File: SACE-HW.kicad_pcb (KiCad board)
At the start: 2 copper layers, 100 x 100 mm, 188 parts, among them IC1 1769205241, J1 1935161, J10 690-005-299-043, J11 Header_Male_Pin_2.54mm_1X4_,_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, J12 XH-4A connector, J13 XH-4A connector, J14 2350514-8, J15 2350514-8, J16 2350514-8, J17 2350514-8, J18 MEM2075-00-140-01-A, J19 2350514-8, J2 2350514-8, J20 2350514-8, J3 Header_Male_Pin_2.54mm_1X2_,_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, J4 XH-4A connector, J5 Header_Male_Pin_2.54mm_1X6_,_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, J6 691317710003, J7 RF1-01K-D-00-50-BK-HDW, J8 RF1-01K-D-00-50-BK-HDW, J9 1935161, Q1 MCB90N12A-TP, Q2 PMV20XNER, Q3 PMV20XNER, Q4 PMV20XNER, Q5 PMV20XNER, Q6 PMV20XNER, Q7 PMV20XNER, SW1 PTS645SM43SMTR92, SW2 PTS645SM43SMTR92, U1 OKI-78SR-5_1.5-W36H-C, U10 ISO7341CQDWQ1, U11 MCP2221A-I_SL, U12 TLA2528IRTER, U13 TLA2528IRTER, U14 TLV9302IDR, U15 MCP4728T-E_UN, U16 74LVC4245APW_118, U2 AZ1117IH-3.3TRG1, U3 AZ1117IH-3.3TRG1, U4 STM32F446RE, U5 MCP6L04T-E/SL, U6 LTV-816S, U7 LTV-816S, U8 TMCS1101A3UQDT, U9 ADC124S021CIMM

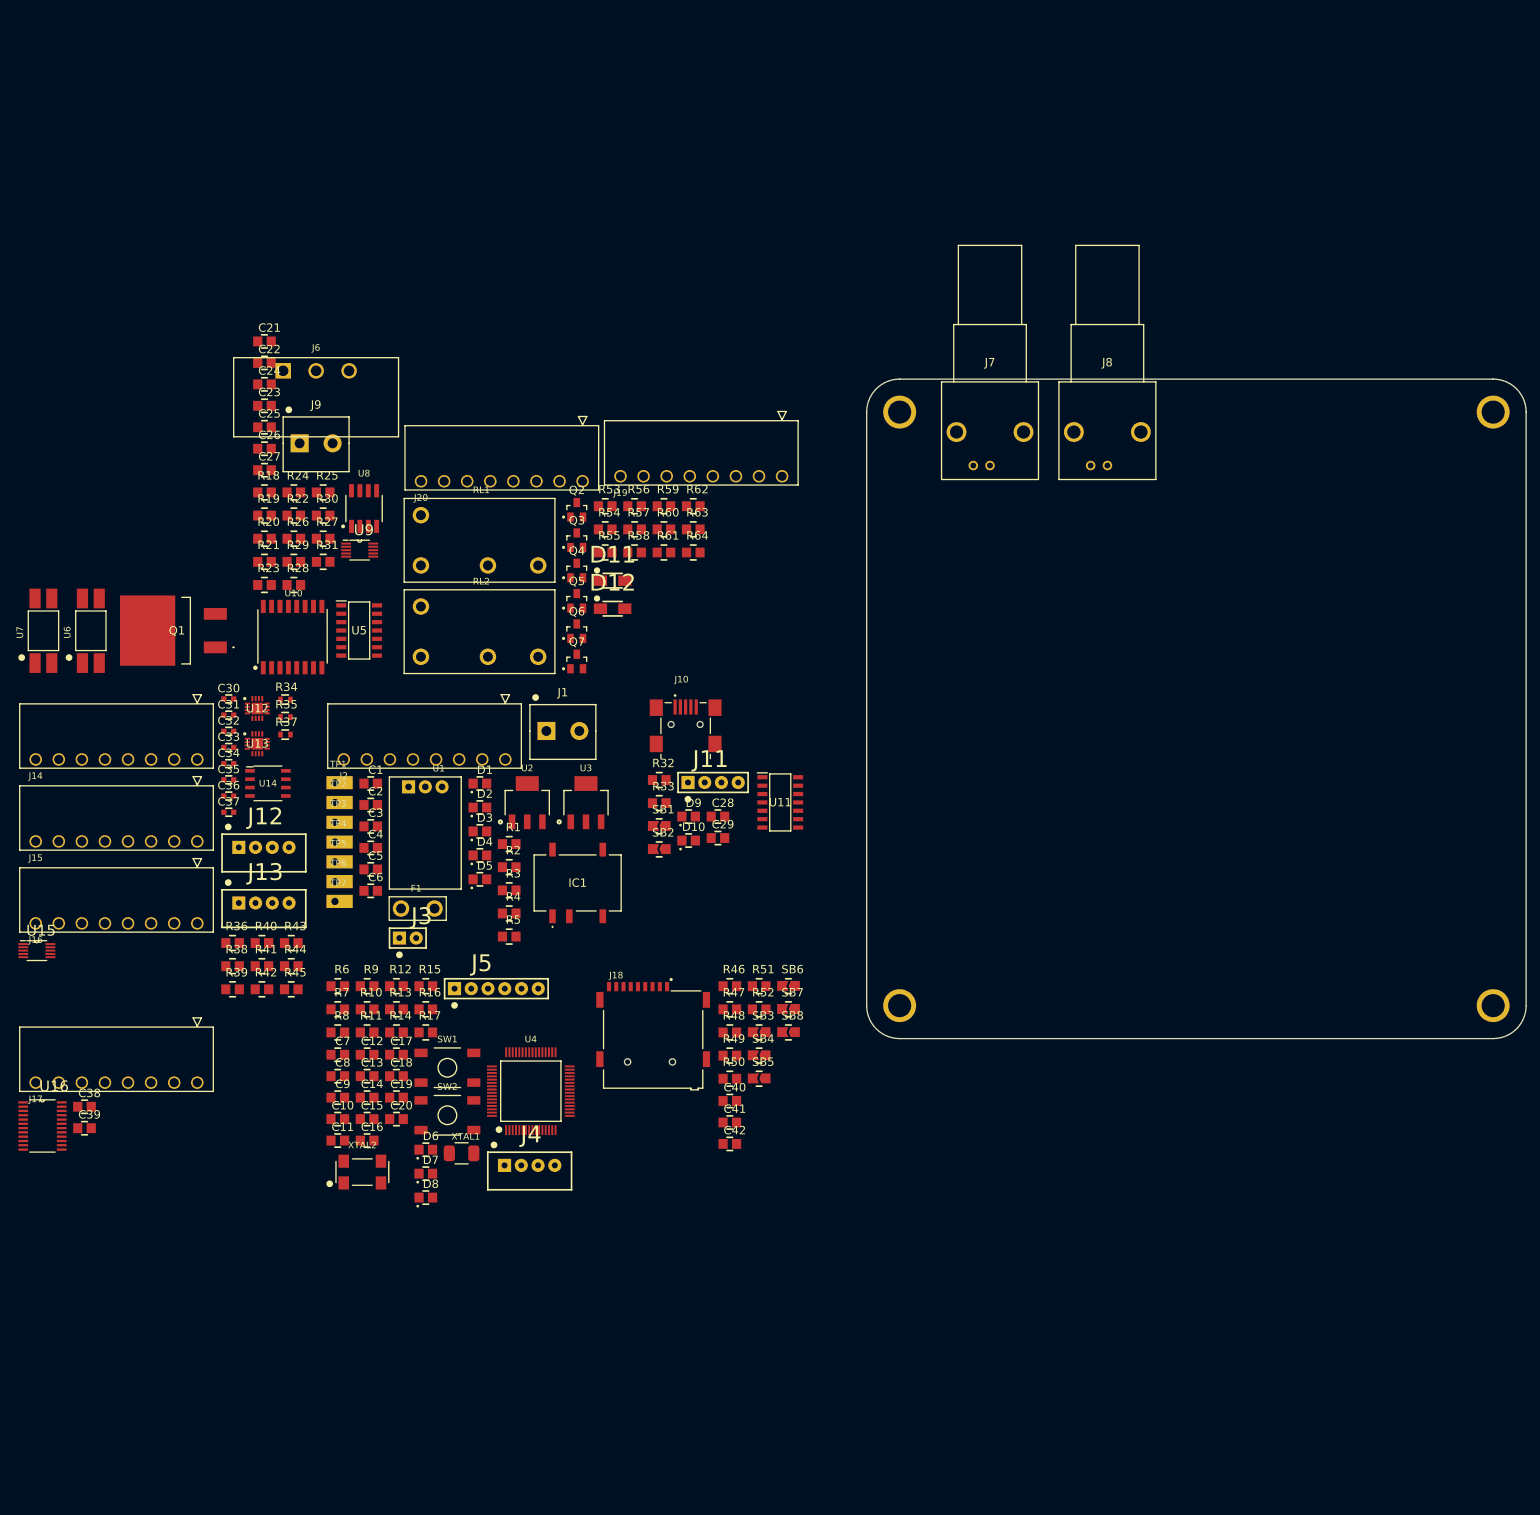
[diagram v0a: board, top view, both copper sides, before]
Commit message: update
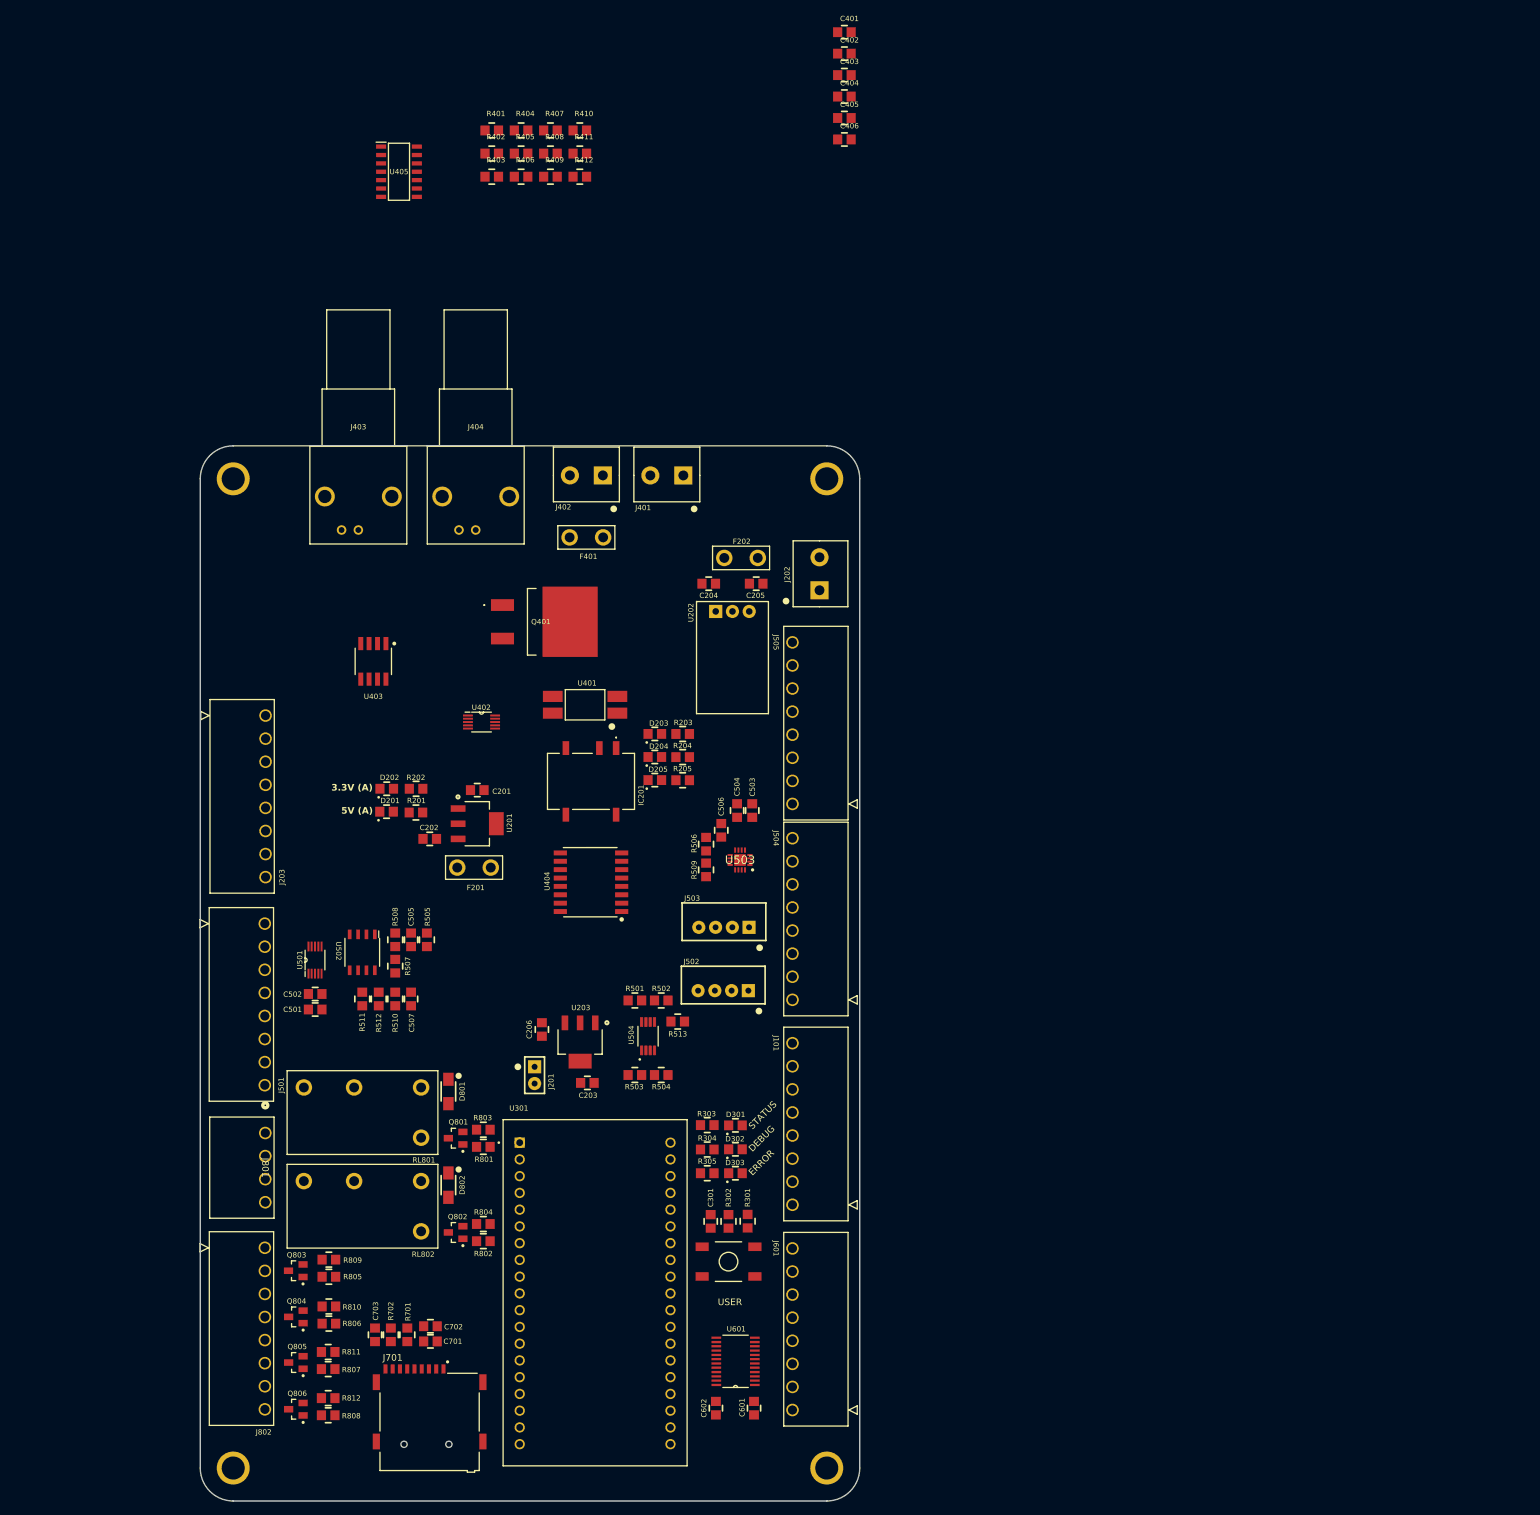
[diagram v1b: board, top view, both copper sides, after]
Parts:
- removed C1, C17, C2: 885012107018, Capacitors:C0805
- removed C10, C13: 885012007027, Capacitors:C0805
- removed C11, C14, C41: 885012107015, Capacitors:C0805
- removed C12: 885012207092, Capacitors:C0805
- removed C15, C16, C18, C19, C20, C22, C23, C26, C28, C29, C38, C39, C40, C42, C8: 885012207098, Capacitors:C0805
- removed C21, C24, C25, C27: 885012207103, Capacitors:C0805
- removed C3, C4: 885012107014, Capacitors:C0805
- removed C30, C31, C32, C33, C34, C35, C36, C37: 885012107015, Capacitors:C0603
- removed C5, C6: 885012107005, Capacitors:C0805
- removed C7, C9: 885012007053, Capacitors:C0805
- removed D1, D2, D3, D4, D5, D6, D9: 150080VS75000, Diodes:LED_0805_GREEN
- removed D10, D7: 150080YS75000, Diodes:LED_0805_YELLOW
- removed D11, D12: DSS16U, Diodes:SOD-123FL
- removed D8: 150080RS75000, Diodes:LED_0805_RED
- removed F1: 39511000440, Fuses:TE5_395
- removed H1, H2, H3, H4: Mounting-Hole-M3, Connectors:Mounting_Hole_3mm
- removed IC1: 1769205241, IC:1769205241
- removed J1, J9: 1935161, Connectors:1935161
- removed J10: 690-005-299-043, Connectors:EDAC_690-005-299-043
- removed J11: Header_Male_Pin_2.54mm_1X4_,_Unshrouded, Connectors:Headers_2.54mm_1X4
- removed J12, J13, J4: XH-4A connector, Connectors:XH-4A
- removed J14, J15, J16, J17, J19, J2, J20: 2350514-8, Connectors:CONN8_2350514-8_TEC
- removed J18: MEM2075-00-140-01-A, Connectors:GCT_MEM2075-00-140-01-A
- removed J3: Header_Male_Pin_2.54mm_1X2_,_Unshrouded, Connectors:Headers_2.54mm_1X2
- removed J5: Header_Male_Pin_2.54mm_1X6_,_Unshrouded, Connectors:Headers_2.54mm_1X6
- removed J6: 691317710003, Connectors:691317710003
- removed J7, J8: RF1-01K-D-00-50-BK-HDW, Connectors:RF101KD0050
- removed Q1: MCB90N12A-TP, IC:MCB90N12ATP
- removed Q2, Q3, Q4, Q5, Q6, Q7: PMV20XNER, IC:SOT-23-3
- removed R1: RC0805JR-0733KL, Resistors:R0805
- removed R10, R9: RC0805JR-07470RL, Resistors:R0805
- removed R11, R36, R7: RC0805JR-070RL, Resistors:R0805
- removed R12, R13, R15, R22, R29, R32, R33, R4, R44, R45, R5: RC0805JR-072K2L, Resistors:R0805
- removed R14, R31, R40, R41, R42, R43, R53, R55, R56, R59, R60, R63: RC0805JR-0710KL, Resistors:R0805
- removed R16, R51, R8: RC0805JR-07150RL, Resistors:R0805
- removed R17, R38, R39, R6: RC0805JR-074K7L, Resistors:R0805
- removed R18, R20: RMCF0805FT10M0, Resistors:R0805
- removed R19, R21: RC0805FR-07200KL, Resistors:R0805
- removed R2, R23, R24, R25, R26, R28, R3, R30: RC0805FR-075K6L, Resistors:R0805
- removed R27, R54, R57, R58, R61, R62, R64: RC0805JR-07330RL, Resistors:R0805
- removed R34, R35, R37: RC0805JR-070RL, Resistors:R0603
- removed R46, R47, R48, R49, R50, R52: RC0805FR-0747KL, Resistors:R0805
- removed RL1, RL2: ALQ312, Relays:ALQ312
- removed SB1, SB2, SB3, SB4, SB5, SB6, SB7, SB8: Solder_Bridge, Connectors:Solder_bridge_0805
- removed SW1, SW2: PTS645SM43SMTR92, Switches:PTS645_6X6X4_SMD
- removed TP1, TP2, TP3, TP4, TP5, TP6, TP7: Test_Point_THM, Connectors:Keystone_5001
- removed U1: OKI-78SR-5_1.5-W36H-C, Assembly:OKI-78SR_Horizontal
- removed U10: ISO7341CQDWQ1, IC:SOIC-16-wide
- removed U11: MCP2221A-I_SL, IC:SOIC127P600X175-14N
- removed U12, U13: TLA2528IRTER, IC:QFN50P300X300X80-17N-D
- removed U14: TLV9302IDR, Assembly:IC8_TLV9302IDR_TEX
- removed U15: MCP4728T-E_UN, IC:SOP50P490X110-10N
- removed U16: 74LVC4245APW_118, IC:SOP65P640X110-24N
- removed U2, U3: AZ1117IH-3.3TRG1, IC:SOT-223-3
- removed U4: STM32F446RE, IC:LQFP-64
- removed U5: MCP6L04T-E/SL, IC:SOIC127P600X175-14N
- removed U6, U7: LTV-816S, IC:4-SMD
- removed U8: TMCS1101A3UQDT, IC:SOIC-8
- removed U9: ADC124S021CIMM, IC:SOP50P490X110-10N
- removed XTAL1: 7A-8.000MAHJ-T, Crystals:TXC_7A_Series
- removed XTAL2: ABS25-32.768KHZ-6-T, Crystals:ABS25
- added C201: 885012107005, Capacitors:C0805, F.Cu at (110.4, 86.1)
- added C202: 885012107014, Capacitors:C0805, F.Cu at (103.2, 93.5)
- added C203: 885012107005, Capacitors:C0805, F.Cu at (129.2, 130.5)
- added C204: 885012107018, Capacitors:C0805, F.Cu at (145.5, 54.8)
- added C205: 885012107018, Capacitors:C0805, F.Cu at (154.8, 54.8)
- added C206: 885012107014, Capacitors:C0805, F.Cu at (121.2, 123.4)
- added C301: 885012207098, Capacitors:C0805, F.Cu at (146.8, 150.5)
- added C401: 885012207098, Capacitors:C0805, F.Cu at (166.1, -28.8)
- added C402: 885012207103, Capacitors:C0805, F.Cu at (166.1, -25.6)
- added C403: 885012207098, Capacitors:C0805, F.Cu at (166.1, -22.3)
- added C404: 885012207103, Capacitors:C0805, F.Cu at (166.1, -19.0)
- added C405: 885012207098, Capacitors:C0805, F.Cu at (166.1, -15.8)
- added C406: 885012207103, Capacitors:C0805, F.Cu at (166.1, -12.5)
- added C501: 885012107015, Capacitors:C0805, F.Cu at (87.9, 119.4)
- added C502: 885012107015, Capacitors:C0805, F.Cu at (87.9, 117.0)
- added C503: 885012107015, Capacitors:C0805, F.Cu at (153.2, 88.2)
- added C504: 885012107015, Capacitors:C0805, F.Cu at (150.8, 88.2)
- added C505: 885012107015, Capacitors:C0805, F.Cu at (101.4, 109.8)
- added C506: 885012107015, Capacitors:C0805, F.Cu at (148.4, 91.2)
- added C507: 885012107015, Capacitors:C0805, F.Cu at (101.4, 118.8)
- added C601: 885012207098, Capacitors:C0805, F.Cu at (153.4, 180.9)
- added C602: 885012207098, Capacitors:C0805, F.Cu at (147.6, 180.9)
- added C701: 885012107015, Capacitors:C0805, F.Cu at (105.4, 169.7)
- added C702: 885012207098, Capacitors:C0805, F.Cu at (103.3, 167.4)
- added C703: 885012207098, Capacitors:C0805, F.Cu at (96.0, 167.7)
- added D201: 150080VS75000, Diodes:LED_0805_GREEN, F.Cu at (96.7, 89.4)
- added D202: 150080VS75000, Diodes:LED_0805_GREEN, F.Cu at (96.7, 85.9)
- added D203: 150080VS75000, Diodes:LED_0805_GREEN, F.Cu at (137.3, 77.6)
- added D204: 150080VS75000, Diodes:LED_0805_GREEN, F.Cu at (137.3, 81.1)
- added D205: 150080VS75000, Diodes:LED_0805_GREEN, F.Cu at (137.3, 84.6)
- added D301: 150080VS75000, Diodes:LED_0805_GREEN, F.Cu at (149.6, 137.0)
- added D302: 150080YS75000, Diodes:LED_0805_YELLOW, F.Cu at (149.6, 140.6)
- added D303: 150080RS75000, Diodes:LED_0805_RED, F.Cu at (149.6, 144.2)
- added D801: DSS16U, Diodes:SOD-123FL, F.Cu at (107.1, 131.8)
- added D802: DSS16U, Diodes:SOD-123FL, F.Cu at (107.1, 146.0)
- added F201: 39511000440, Fuses:TE5_395, F.Cu at (111.0, 97.9)
- added F202: 39511000440, Fuses:TE5_395, F.Cu at (151.4, 50.9)
- added F401: 0698Q6300-01, Fuses:TE5_395, F.Cu at (128.0, 47.8)
- added H101: Mounting-Hole-M3, Connectors:Mounting_Hole_3mm, F.Cu at (164.4, 188.9)
- added H102: Mounting-Hole-M3, Connectors:Mounting_Hole_3mm, F.Cu at (164.4, 38.9)
- added H103: Mounting-Hole-M3, Connectors:Mounting_Hole_3mm, F.Cu at (74.5, 38.9)
- added H104: Mounting-Hole-M3, Connectors:Mounting_Hole_3mm, F.Cu at (74.5, 188.9)
- added IC201: 1769205241, IC:1769205241, F.Cu at (128.7, 84.8)
- added J101: 2350514-8, Connectors:CONN8_2350514-8_TEC, F.Cu at (159.2, 149.0)
- added J201: Header_Male_Pin_2.54mm_1X2_,_Unshrouded, Connectors:Headers_2.54mm_1X2, F.Cu at (120.2, 128.1)
- added J202: 1935161, Connectors:1935161, F.Cu at (163.3, 53.3)
- added J203: 2350514-8, Connectors:CONN8_2350514-8_TEC, F.Cu at (79.3, 74.8)
- added J401: 1935161, Connectors:1935161, F.Cu at (140.2, 38.4)
- added J402: 1935161, Connectors:1935161, F.Cu at (128.0, 38.4)
- added J403: RF1-01K-D-00-50-BK-HDW, Connectors:RF101KD0050, F.Cu at (93.4, 46.7)
- added J404: RF1-01K-D-00-50-BK-HDW, Connectors:RF101KD0050, F.Cu at (111.2, 46.7)
- added J501: 2350514-8, Connectors:CONN8_2350514-8_TEC, F.Cu at (79.2, 106.4)
- added J502: XH-4A connector, Connectors:XH-4A, F.Cu at (152.6, 116.5)
- added J503: XH-4A connector, Connectors:XH-4A, F.Cu at (152.7, 106.9)
- added J504: 2350514-8, Connectors:CONN8_2350514-8_TEC, F.Cu at (159.2, 117.9)
- added J505: 2350514-8, Connectors:CONN8_2350514-8_TEC, F.Cu at (159.2, 88.2)
- added J601: 2350514-8, Connectors:CONN8_2350514-8_TEC, F.Cu at (159.2, 180.1)
- added J701: MEM2075-00-140-01-A, Connectors:GCT_MEM2075-00-140-01-A, F.Cu at (103.8, 185.3)
- added J801: 2350514-4, Connectors:CONN4_1155650000_TEC, F.Cu at (79.3, 138.1)
- added J802: 2350514-8, Connectors:CONN8_2350514-8_TEC, F.Cu at (79.2, 155.5)
- added Q401: MCB90N12A-TP, IC:MCB90N12ATP, F.Cu at (123.5, 60.6)
- added Q801: PMV20XNER, IC:SOT-23-3, F.Cu at (108.2, 138.9)
- added Q802: PMV20XNER, IC:SOT-23-3, F.Cu at (108.2, 153.2)
- added Q803: PMV20XNER, IC:SOT-23-3, F.Cu at (83.9, 159.0)
- added Q804: PMV20XNER, IC:SOT-23-3, F.Cu at (84.0, 166.0)
- added Q805: PMV20XNER, IC:SOT-23-3, F.Cu at (84.0, 172.9)
- added Q806: PMV20XNER, IC:SOT-23-3, F.Cu at (84.0, 180.0)
- added R201: RC0805FR-075K6L, Resistors:R0805, F.Cu at (101.1, 89.5)
- added R202: RC0805JR-072K2L, Resistors:R0805, F.Cu at (101.2, 85.9)
- added R203: RC0805JR-0733KL, Resistors:R0805, F.Cu at (141.6, 77.6)
- added R204: RC0805FR-075K6L, Resistors:R0805, F.Cu at (141.6, 81.1)
- added R205: RC0805JR-072K2L, Resistors:R0805, F.Cu at (141.6, 84.6)
- added R301: RC0805JR-074K7L, Resistors:R0805, F.Cu at (152.4, 152.5)
- added R302: RC0805JR-07150RL, Resistors:R0805, F.Cu at (149.6, 150.5)
- added R303: RC0805JR-072K2L, Resistors:R0805, F.Cu at (145.3, 136.9)
- added R304: RC0805JR-072K2L, Resistors:R0805, F.Cu at (145.3, 140.6)
- added R305: RC0805JR-072K2L, Resistors:R0805, F.Cu at (145.3, 144.2)
- added R401: RC0805JR-0710KL, Resistors:R0805, F.Cu at (112.6, -13.9)
- added R402: RC0805JR-07330RL, Resistors:R0805, F.Cu at (112.6, -10.4)
- added R403: RC0805JR-072K2L, Resistors:R0805, F.Cu at (112.6, -6.89)
- added R404: RC0805FR-075K6L, Resistors:R0805, F.Cu at (117.1, -13.9)
- added R405: ERJ-6ENF1404V, Resistors:R0805, F.Cu at (117.1, -10.4)
- added R406: RC0805JR-0710KL, Resistors:R0805, F.Cu at (117.1, -6.89)
- added R407: RC0805JR-0710KL, Resistors:R0805, F.Cu at (121.5, -13.9)
- added R408: RC0805FR-0747KL, Resistors:R0805, F.Cu at (121.5, -10.4)
- added R409: RC0805JR-0710KL, Resistors:R0805, F.Cu at (121.5, -6.89)
- added R410: ERJ-6ENF1404V, Resistors:R0805, F.Cu at (126.0, -13.9)
- added R411: RC0805JR-0710KL, Resistors:R0805, F.Cu at (126.0, -10.4)
- added R412: RC0805FR-0747KL, Resistors:R0805, F.Cu at (126.0, -6.89)
- added R501: RC0805JR-074K7L, Resistors:R0805, F.Cu at (136.4, 118.0)
- added R502: RC0805JR-074K7L, Resistors:R0805, F.Cu at (138.3, 118.0)
- added R503: RC0805JR-074K7L, Resistors:R0805, F.Cu at (136.4, 129.3)
- added R504: RC0805JR-074K7L, Resistors:R0805, F.Cu at (138.3, 129.3)
- added R505: RC0805JR-072K2L, Resistors:R0805, F.Cu at (103.8, 109.8)
- added R506: 0hms_0.5W, Resistors:R0805, F.Cu at (146.2, 93.3)
- added R507: RC0805JR-0710KL, Resistors:R0805, F.Cu at (99.0, 113.8)
- added R508: RC0805JR-0710KL, Resistors:R0805, F.Cu at (99.0, 109.8)
- added R509: 0hms_0.5W, Resistors:R0805, F.Cu at (146.2, 97.2)
- added R510: RC0805JR-072K2L, Resistors:R0805, F.Cu at (99.0, 118.8)
- added R511: RC0805JR-0710KL, Resistors:R0805, F.Cu at (94.0, 118.8)
- added R512: RC0805JR-0710KL, Resistors:R0805, F.Cu at (96.5, 118.8)
- added R513: RC0805JR-0710KL, Resistors:R0805, F.Cu at (142.9, 121.2)
- added R701: RC0805FR-0747KL, Resistors:R0805, F.Cu at (100.8, 167.7)
- added R702: RC0805JR-07150RL, Resistors:R0805, F.Cu at (98.3, 169.7)
- added R801: RC0805JR-07330RL, Resistors:R0805, F.Cu at (113.4, 140.2)
- added R802: RC0805JR-07330RL, Resistors:R0805, F.Cu at (113.4, 154.5)
- added R803: RC0805JR-0710KL, Resistors:R0805, F.Cu at (111.3, 137.6)
- added R804: RC0805JR-0710KL, Resistors:R0805, F.Cu at (111.3, 151.9)
- added R805: RC0805JR-07330RL, Resistors:R0805, F.Cu at (90.0, 159.9)
- added R806: RC0805JR-07330RL, Resistors:R0805, F.Cu at (90.0, 167.0)
- added R807: RC0805JR-07330RL, Resistors:R0805, F.Cu at (89.9, 173.9)
- added R808: RC0805JR-07330RL, Resistors:R0805, F.Cu at (89.9, 180.9)
- added R809: RC0805JR-0710KL, Resistors:R0805, F.Cu at (87.9, 157.3)
- added R810: RC0805JR-0710KL, Resistors:R0805, F.Cu at (87.9, 164.4)
- added R811: RC0805JR-0710KL, Resistors:R0805, F.Cu at (87.8, 171.3)
- added R812: RC0805JR-0710KL, Resistors:R0805, F.Cu at (87.8, 178.3)
- added RL801: ALQ312, Relays:ALQ312, F.Cu at (94.0, 135.0)
- added RL802: ALQ312, Relays:ALQ312, F.Cu at (94.0, 149.2)
- added SW301: PTS645SM43SMTR92, Switches:PTS645_6X6X4_SMD, F.Cu at (149.6, 157.6)
- added U201: AZ1117IH-3.3TRG1, IC:SOT-223-3, F.Cu at (111.5, 91.2)
- added U202: OKI-78SR-5_1.5-W36H-C, Assembly:OKI-78SR_Horizontal, F.Cu at (150.2, 59.0)
- added U203: AZ1117IH-3.3TRG1, IC:SOT-223-3, F.Cu at (127.0, 124.3)
- added U301: ESP32-DEVKITC-32D, Assembly:MODULE_ESP32-DEVKITC-32D, F.Cu at (129.3, 159.3)
- added U401: LTV-816S, IC:4-SMD, F.Cu at (127.8, 73.2)
- added U402: ADC124S021CIMM, IC:SOP50P490X110-10N, F.Cu at (112.1, 75.8)
- added U403: TMCS1101A3UQDT, IC:SOIC-8, F.Cu at (95.7, 66.6)
- added U404: ISO7341CQDWQ1, IC:SOIC-16-wide, F.Cu at (125.2, 100.1)
- added U405: MCP6L04T-E/SL, IC:SOIC127P600X175-14N, F.Cu at (99.6, -7.64)
- added U501: MCP4728T-E_UN, IC:SOP50P490X110-10N, F.Cu at (86.8, 111.9)
- added U502: TLV9302IDR, Assembly:IC8_TLV9302IDR_TEX, F.Cu at (94.0, 110.7)
- added U503: TLA2528IRTER, IC:QFN50P300X300X80-17N-D, F.Cu at (151.3, 96.7)
- added U504: TCA9617BDGKR, IC:SOP65P490X110-8N, F.Cu at (137.3, 123.4)
- added U601: 74LVC4245APW_118, IC:SOP65P640X110-24N, F.Cu at (150.6, 172.7)
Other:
- board size 100 x 100 mm -> 100 x 160 mm
- board text added: "3.3V (A)"
- board text added: "5V (A)"
- board text added: "DEBUG"
- board text added: "ERROR"
- board text added: "STATUS"
- board text added: "USER"
